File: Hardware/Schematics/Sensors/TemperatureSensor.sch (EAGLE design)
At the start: 6 parts, among them IC1 DS18B20

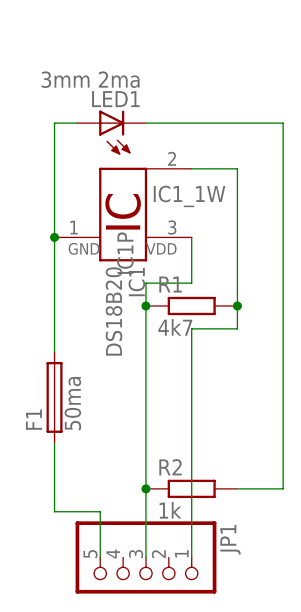
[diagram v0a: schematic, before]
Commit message: sensors
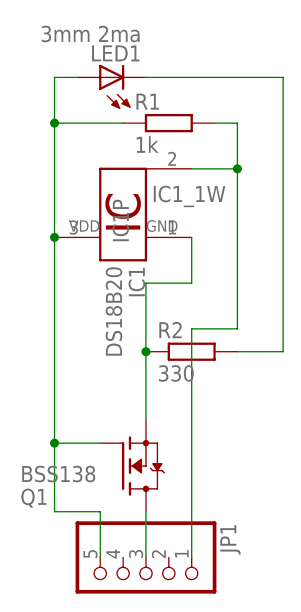
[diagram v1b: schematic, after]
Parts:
- removed F1: 50ma, fuse:MF-SMDF050
- added Q1: BSS138, Cing Library:BSS138
- JP1: device pinhead:PINHD-1X5/90 -> pinhead:PINHD-1X5
- R1: value 4k7 -> 1k
- R2: value 1k -> 330
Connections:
- removed net N$14: IC1P.VDD, JP1.3, R1.1, R2.1
- removed net N$15: F1.1, JP1.5
- new net N$3: JP1.3, Q1.D
- new net N$4: IC1P.GND, Q1.S, R2.1
- net N$1: now also IC1P.VDD, JP1.5, Q1.G, R1.1; no longer F1.2, IC1P.GND
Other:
- moved on the sheet: IC1P, LED1, R1, R2
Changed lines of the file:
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@@
 <layer number="59" name="tCarbon" color="7" fill="1" visible="no" active="no"/>
 <layer number="60" name="bCarbon" color="7" fill="1" visible="no" active="no"/>
+<layer number="88" name="SimResults" color="9" fill="1" visible="yes" active="yes"/>
+<layer number="89" name="SimProbes" color="9" fill="1" visible="yes" active="yes"/>
 <layer number="90" name="Modules" color="5" fill="1" visible="yes" active="yes"/>
 <layer number="91" name="Nets" color="2" fill="1" visible="yes" active="yes"/>
@@
 <layer number="112" name="tSilk" color="7" fill="1" visible="no" active="yes"/>
 <layer number="113" name="ReferenceLS" color="7" fill="1" visible="no" active="no"/>
+<layer number="114" name="Badge_Outline" color="7" fill="1" visible="yes" active="yes"/>
+<layer number="115" name="ReferenceISLANDS" color="7" fill="1" visible="yes" active="yes"/>
 <layer number="116" name="Patch_BOT" color="9" fill="4" visible="no" active="yes"/>
+<layer number="117" name="BACKMAAT1" color="7" fill="1" visible="no" active="no"/>
 <layer number="118" name="Rect_Pads" color="7" fill="1" visible="no" active="no"/>
+<layer number="119" name="KAP_TEKEN" color="7" fill="1" visible="no" active="no"/>
+<layer number="120" name="KAP_MAAT1" color="7" fill="1" visible="no" active="no"/>
 <layer number="121" name="_tsilk" color="7" fill="1" visible="no" active="yes"/>
 <layer number="122" name="_bsilk" color="7" fill="1" visible="no" active="yes"/>
@@
 <layer number="128" name="_bValues" color="7" fill="1" visible="no" active="yes"/>
 <layer number="129" name="Mask" color="7" fill="1" visible="yes" active="yes"/>
+<layer number="130" name="SMDSTROOK" color="7" fill="1" visible="no" active="no"/>
 <layer number="131" name="tAdjust" color="7" fill="1" visible="no" active="yes"/>
 <layer number="132" name="bAdjust" color="7" fill="1" visible="no" active="yes"/>
+<layer number="133" name="bottom_silk" color="7" fill="1" visible="yes" active="yes"/>
+<layer number="134" name="silk_top" color="7" fill="1" visible="no" active="no"/>
+<layer number="135" name="silk_bottom" color="7" fill="1" visible="no" active="no"/>
+<layer number="136" name="silktop" color="7" fill="1" visible="yes" active="yes"/>
+<layer number="137" name="silkbottom" color="7" fill="1" visible="yes" active="yes"/>
 <layer number="144" name="Drill_legend" color="7" fill="1" visible="no" active="yes"/>
+<layer number="145" name="DrillLegend_01-16" color="7" fill="1" visible="yes" active="yes"/>
+<layer number="146" name="DrillLegend_01-20" color="7" fill="1" visible="yes" active="yes"/>
 <layer number="150" name="Notes" color="7" fill="1" visible="no" active="yes"/>
 <layer number="151" name="HeatSink" color="7" fill="1" visible="no" active="yes"/>
@@
 </classes>
 <parts>
-<part name="F1" library="fuse" deviceset="MF-SMDF" device="" technology="050" value="50ma"/>
 <part name="LED1" library="led" deviceset="TLLY4400" device="" value="3mm 2ma"/>
-<part name="R2" library="rcl" deviceset="R-EU_" device="R1206" value="1k"/>
+<part name="R2" library="rcl" deviceset="R-EU_" device="R1206" value="330"/>
 <part name="IC1" library="1wire" deviceset="DS18B20" device=""/>
-<part name="R1" library="rcl" deviceset="R-EU_" device="R1206" value="4k7"/>
-<part name="JP1" library="pinhead" library_urn="urn:adsk.eagle:library:325" deviceset="PINHD-1X5" device="/90" package3d_urn="urn:adsk.eagle:package:22467/2"/>
+<part name="R1" library="rcl" deviceset="R-EU_" device="R1206" value="1k"/>
+<part name="JP1" library="pinhead" library_urn="urn:adsk.eagle:library:325" deviceset="PINHD-1X5" device="" package3d_urn="urn:adsk.eagle:package:22469/2"/>
+<part name="Q1" library="Cing Library" deviceset="BSS138" device=""/>
 </parts>
 <sheets>
@@
 </plain>
 <instances>
-<instance part="F1" gate="A" x="7.62" y="25.4" rot="R90"/>
-<instance part="LED1" gate="G$1" x="12.7" y="55.88" rot="R90"/>
-<instance part="R2" gate="G$1" x="22.86" y="15.24"/>
+<instance part="LED1" gate="G$1" x="12.7" y="60.96" rot="R90"/>
+<instance part="R2" gate="G$1" x="22.86" y="30.48"/>
 <instance part="IC1" gate="A" x="15.24" y="45.72" rot="R270"/>
 <instance part="IC1" gate="_1W" x="17.78" y="50.8" rot="R180"/>
-<instance part="IC1" gate="P" x="15.24" y="43.18" rot="R270"/>
-<instance part="R1" gate="G$1" x="22.86" y="35.56"/>
+<instance part="IC1" gate="P" x="15.24" y="43.18" rot="R90"/>
+<instance part="R1" gate="G$1" x="20.32" y="55.88"/>
 <instance part="JP1" gate="A" x="17.78" y="5.08" rot="R270"/>
+<instance part="Q1" gate="G$1" x="15.24" y="17.78" rot="MR180"/>
 </instances>
 <busses>
 </busses>
 <nets>
-<net name="N$14" class="0">
-<segment>
-<pinref part="R2" gate="G$1" pin="1"/>
-<wire x1="17.78" y1="15.24" x2="17.78" y2="7.62" width="0.1524" layer="91"/>
-<junction x="17.78" y="15.24"/>
-<wire x1="17.78" y1="15.24" x2="17.78" y2="35.56" width="0.1524" layer="91"/>
-<pinref part="IC1" gate="P" pin="VDD"/>
-<wire x1="17.78" y1="35.56" x2="17.78" y2="38.1" width="0.1524" layer="91"/>
-<wire x1="17.78" y1="38.1" x2="22.86" y2="38.1" width="0.1524" layer="91"/>
-<wire x1="22.86" y1="38.1" x2="22.86" y2="43.18" width="0.1524" layer="91"/>
-<pinref part="R1" gate="G$1" pin="1"/>
-<junction x="17.78" y="35.56"/>
-<pinref part="JP1" gate="A" pin="3"/>
-</segment>
-</net>
-<net name="N$15" class="0">
+<net name="N$1" class="0">
 <segment>
 <wire x1="7.62" y1="12.7" x2="12.7" y2="12.7" width="0.1524" layer="91"/>
 <wire x1="12.7" y1="12.7" x2="12.7" y2="7.62" width="0.1524" layer="91"/>
-<pinref part="F1" gate="A" pin="1"/>
 <wire x1="7.62" y1="20.32" x2="7.62" y2="12.7" width="0.1524" layer="91"/>
 <pinref part="JP1" gate="A" pin="5"/>
-</segment>
-</net>
-<net name="N$1" class="0">
-<segment>
-<pinref part="F1" gate="A" pin="2"/>
+<wire x1="7.62" y1="30.48" x2="7.62" y2="20.32" width="0.1524" layer="91"/>
 <pinref part="LED1" gate="G$1" pin="A"/>
-<wire x1="10.16" y1="55.88" x2="7.62" y2="55.88" width="0.1524" layer="91"/>
-<wire x1="7.62" y1="55.88" x2="7.62" y2="43.18" width="0.1524" layer="91"/>
+<wire x1="10.16" y1="60.96" x2="7.62" y2="60.96" width="0.1524" layer="91"/>
+<wire x1="7.62" y1="30.48" x2="7.62" y2="43.18" width="0.1524" layer="91"/>
+<pinref part="IC1" gate="P" pin="VDD"/>
+<wire x1="7.62" y1="43.18" x2="7.62" y2="55.88" width="0.1524" layer="91"/>
+<junction x="7.62" y="43.18"/>
+<pinref part="R1" gate="G$1" pin="1"/>
+<wire x1="7.62" y1="55.88" x2="7.62" y2="60.96" width="0.1524" layer="91"/>
+<wire x1="15.24" y1="55.88" x2="7.62" y2="55.88" width="0.1524" layer="91"/>
+<junction x="7.62" y="55.88"/>
+<pinref part="Q1" gate="G$1" pin="G"/>
+<wire x1="12.7" y1="20.32" x2="7.62" y2="20.32" width="0.1524" layer="91"/>
+<junction x="7.62" y="20.32"/>
+</segment>
+</net>
+<net name="N$2" class="0">
+<segment>
+<pinref part="LED1" gate="G$1" pin="C"/>
+<wire x1="33.02" y1="60.96" x2="17.78" y2="60.96" width="0.1524" layer="91"/>
+<pinref part="R2" gate="G$1" pin="2"/>
+<wire x1="27.94" y1="30.48" x2="33.02" y2="30.48" width="0.1524" layer="91"/>
+<wire x1="33.02" y1="30.48" x2="33.02" y2="60.96" width="0.1524" layer="91"/>
+</segment>
+</net>
+<net name="N$4" class="0">
+<segment>
 <pinref part="IC1" gate="P" pin="GND"/>
-<wire x1="7.62" y1="43.18" x2="7.62" y2="30.48" width="0.1524" layer="91"/>
-<junction x="7.62" y="43.18"/>
-</segment>
-</net>
-<net name="N$2" class="0">
-<segment>
-<pinref part="LED1" gate="G$1" pin="C"/>
-<wire x1="33.02" y1="55.88" x2="17.78" y2="55.88" width="0.1524" layer="91"/>
-<pinref part="R2" gate="G$1" pin="2"/>
-<wire x1="27.94" y1="15.24" x2="33.02" y2="15.24" width="0.1524" layer="91"/>
-<wire x1="33.02" y1="15.24" x2="33.02" y2="55.88" width="0.1524" layer="91"/>
-</segment>
-</net>
-<net name="N$3" class="0">
+<wire x1="22.86" y1="38.1" x2="22.86" y2="43.18" width="0.1524" layer="91"/>
+<pinref part="R2" gate="G$1" pin="1"/>
+<wire x1="22.86" y1="38.1" x2="17.78" y2="38.1" width="0.1524" layer="91"/>
+<wire x1="17.78" y1="38.1" x2="17.78" y2="30.48" width="0.1524" layer="91"/>
+<pinref part="Q1" gate="G$1" pin="S"/>
+<wire x1="17.78" y1="22.86" x2="17.78" y2="30.48" width="0.1524" layer="91"/>
+<junction x="17.78" y="30.48"/>
+</segment>
+</net>
+<net name="N$5" class="0">
 <segment>
 <pinref part="IC1" gate="_1W" pin="1W"/>
+<wire x1="27.94" y1="50.8" x2="22.86" y2="50.8" width="0.1524" layer="91"/>
 <wire x1="22.86" y1="7.62" x2="22.86" y2="33.02" width="0.1524" layer="91"/>
 <wire x1="22.86" y1="33.02" x2="27.94" y2="33.02" width="0.1524" layer="91"/>
-<wire x1="27.94" y1="33.02" x2="27.94" y2="35.56" width="0.1524" layer="91"/>
-<wire x1="27.94" y1="35.56" x2="27.94" y2="50.8" width="0.1524" layer="91"/>
-<wire x1="27.94" y1="50.8" x2="22.86" y2="50.8" width="0.1524" layer="91"/>
+<pinref part="JP1" gate="A" pin="1"/>
+<wire x1="27.94" y1="50.8" x2="27.94" y2="33.02" width="0.1524" layer="91"/>
 <pinref part="R1" gate="G$1" pin="2"/>
-<junction x="27.94" y="35.56"/>
-<pinref part="JP1" gate="A" pin="1"/>
-</segment>
-</net>
+<wire x1="27.94" y1="50.8" x2="27.94" y2="55.88" width="0.1524" layer="91"/>
+<wire x1="27.94" y1="55.88" x2="25.4" y2="55.88" width="0.1524" layer="91"/>
+<junction x="27.94" y="50.8"/>
+</segment>
+</net>
+<net name="N$3" class="0">
+<segment>
+<pinref part="Q1" gate="G$1" pin="D"/>
+<pinref part="JP1" gate="A" pin="3"/>
+<wire x1="17.78" y1="12.7" x2="17.78" y2="7.62" width="0.1524" layer="91"/>
+</segment>
+</net>
